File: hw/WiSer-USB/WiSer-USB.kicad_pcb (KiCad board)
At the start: 4 copper layers, 25.8 x 14.4 mm, 48 parts, among them P1 USB_C_Plug, U1 AP2112K-3.3TRG1, U2 USBLC6-2P6, U3 ESP32-S2, Y1 40MHz

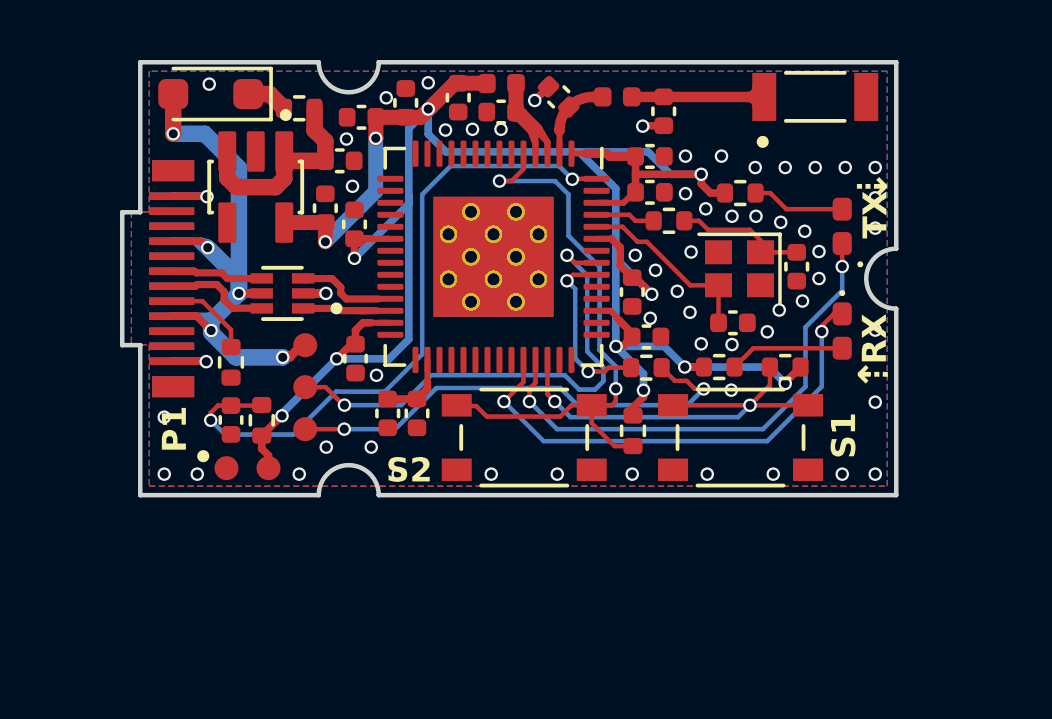
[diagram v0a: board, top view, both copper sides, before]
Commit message: Update hardware design files
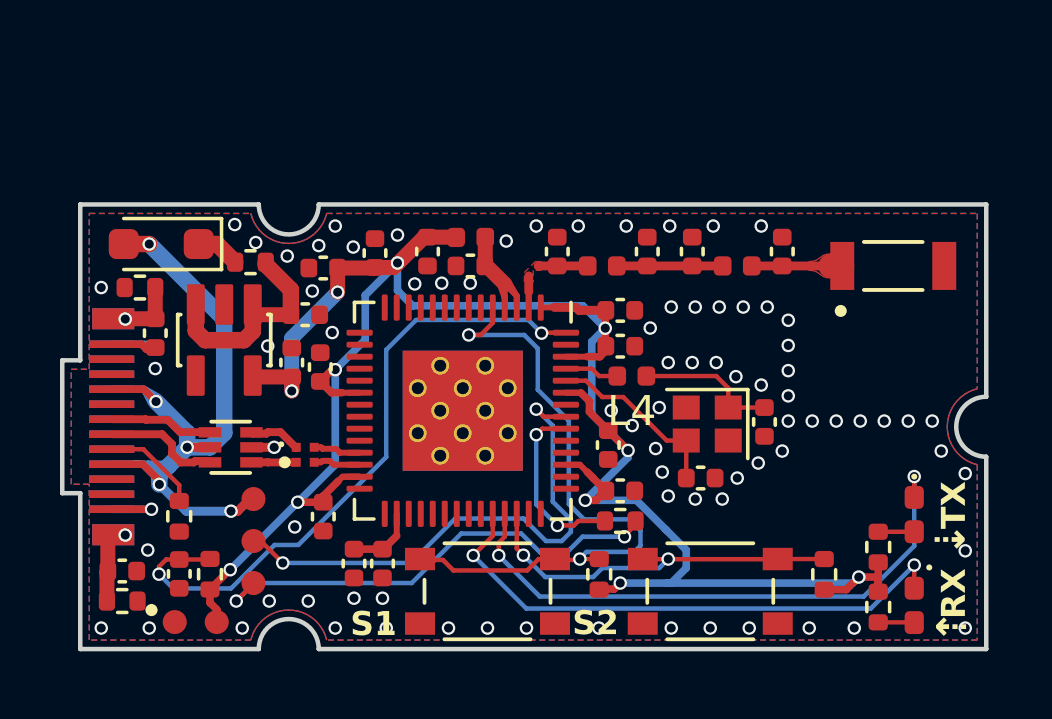
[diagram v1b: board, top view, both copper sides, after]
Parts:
- removed the C18 at (106.0, 81.6)
- added C1: 0.1u, Capacitor_SMD:C_0402_1005Metric, F.Cu at (92.5, 89.5)
- added C17: TBD, Capacitor_SMD:C_0402_1005Metric, F.Cu at (113.4, 86.8)
- added C19: TBD, Capacitor_SMD:C_0402_1005Metric, F.Cu at (110.4, 86.8)
- added C2: 0.1u, Capacitor_SMD:C_0402_1005Metric, F.Cu at (91.4, 97.4)
- added C23: TBD, Capacitor_SMD:C_0402_1005Metric, F.Cu at (105.9, 86.8)
- added L2: L_Ferrite_Coupled_Small_1243, DLM0NSM900HY2D:FIL_DLM0NSM900HY2D, F.Cu at (97.5, 93.5)
- added L3: TBD, Inductor_SMD:L_0402_1005Metric, F.Cu at (111.9, 87.2)
- added L4: 24n, Inductor_SMD:L_0402_1005Metric, F.Cu at (108.4, 90.9)
- added R1: 330, Resistor_SMD:R_0402_1005Metric, F.Cu at (92.0, 88.0)
- R2: value 22 -> 330
- S1: value USER -> BOOT
- S2: value BOOT -> USER
- moved R2 22.2 mm to (91.4, 98.4), turned to 0 degrees
- moved R7 14.5 mm to (116.6, 98.6), turned to 90 degrees
- moved D2 12.9 mm to (117.8, 98.5), turned to -90 degrees
- moved S1 9.87 mm to (103.6, 98.1)
- moved G*** 8.25 mm to (96.6, 92.6)
- moved S2 8.04 mm to (111.0, 98.1)
- moved R8 8.01 mm to (116.6, 96.6), turned to -90 degrees
- moved R9 7.03 mm to (114.8, 97.5), turned to 90 degrees
- moved D3 6.57 mm to (117.8, 95.5)
- moved G*** 6.35 mm to (114.8, 91.6)
- moved E1 6.21 mm to (117.1, 87.2)
- moved L5 5.66 mm to (107.4, 87.2)
- moved C21 5.41 mm to (93.3, 97.5)
- moved R3 5.41 mm to (93.3, 95.6)
- moved TP4 5.41 mm to (95.8, 96.4)
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- renumbered C8 to C10, C9 to C11, C10 to C12, C11 to C13, C12 to C14, C13 to C15, C14 to C16, C15 to C18, C16 to C20, C19 to C21, C17 to C22, C1 to C3, C2 to C4, C3 to C5, C4 to C6, C5 to C7, C6 to C8, C7 to C9, L2 to L5, R1 to R3, R3 to R4, R4 to R5, R8 to R6, R6 to R7, R7 to R8, R5 to R9
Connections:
- C20 pad 1: Net-(C16-Pad1) -> Net-(C20-Pad1)
- C22 pad 1: Net-(C17-Pad1) -> Net-(C19-Pad1)
- D2 pad 1: /LED_TXD -> /LED_RXD
- D3 pad 1: /LED_RXD -> /LED_TXD
- L5 pad 2: Net-(C17-Pad1) -> Net-(C19-Pad1)
- P1 pad S1: unconnected-(P1-SHIELD-PadS1) -> Net-(P1-SHIELD)
- R2 pad 1: Net-(C16-Pad1) -> Net-(P1-SHIELD)
- R2 pad 2: /XTAL_P -> GND
- S1 pad 3: /USER_IN -> /BOOT
- S1 pad 4: /USER_IN -> /BOOT
- S2 pad 3: /BOOT -> /USER_IN
- S2 pad 4: /BOOT -> /USER_IN
- U3 pad 25: /USB- -> /USB_FIL-
- U3 pad 26: /USB+ -> /USB_FIL+
- Y1 pad 1: Net-(C16-Pad1) -> Net-(C20-Pad1)
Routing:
- net +5V: track 22.6 -> 27.9 mm
- net Net-(P1-SHIELD): track 0.00 -> 4.75 mm, vias 0 -> 2
- net Net-(C20-Pad1): track 0.00 -> 4.71 mm
- net Net-(C16-Pad1): track 4.42 -> 0.00 mm
- net Net-(C19-Pad1): track 0.00 -> 3.56 mm
- net +3V3: track 77.2 -> 74.4 mm, vias 12 -> 11
- net /LED_TXD: track 16.9 -> 19.7 mm
- net Net-(D3-A): track 3.85 -> 1.22 mm
- net Net-(D2-A): track 3.11 -> 1.05 mm
- net /LED_RXD: track 16.4 -> 18.5 mm
- net /BOOT: track 19.5 -> 21.4 mm
- net /USB_FIL-: track 0.00 -> 1.59 mm
- net /USB_FIL+: track 0.00 -> 1.59 mm
- net /USER_IN: track 14.4 -> 12.9 mm
- net Net-(C17-Pad1): track 4.41 -> 3.02 mm
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- added copper zone on F.Cu, net /LNA_IN
- added copper zone on F.Cu, net Net-(C17-Pad1)
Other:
- board size 25.8 x 14.4 mm -> 30.8 x 14.8 mm
- board text added: "Rev-1.2"
- board text removed: "P1"
- board text removed: "Rev-1.1"
